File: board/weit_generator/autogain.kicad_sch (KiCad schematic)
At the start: 19 parts, among them Q1 BC547

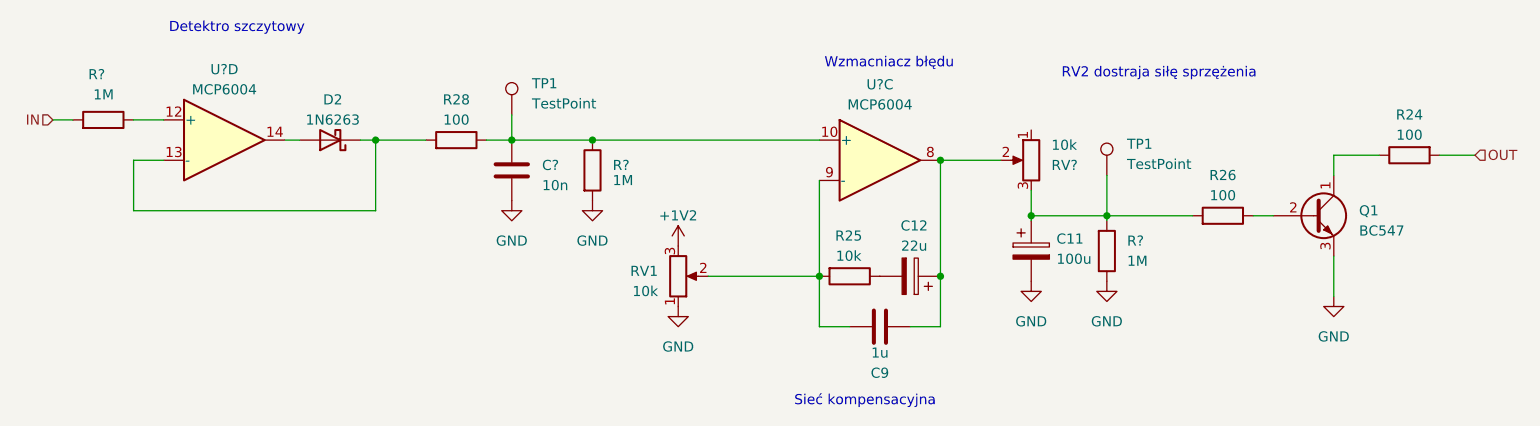
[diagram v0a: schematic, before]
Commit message: Final revision - submitting
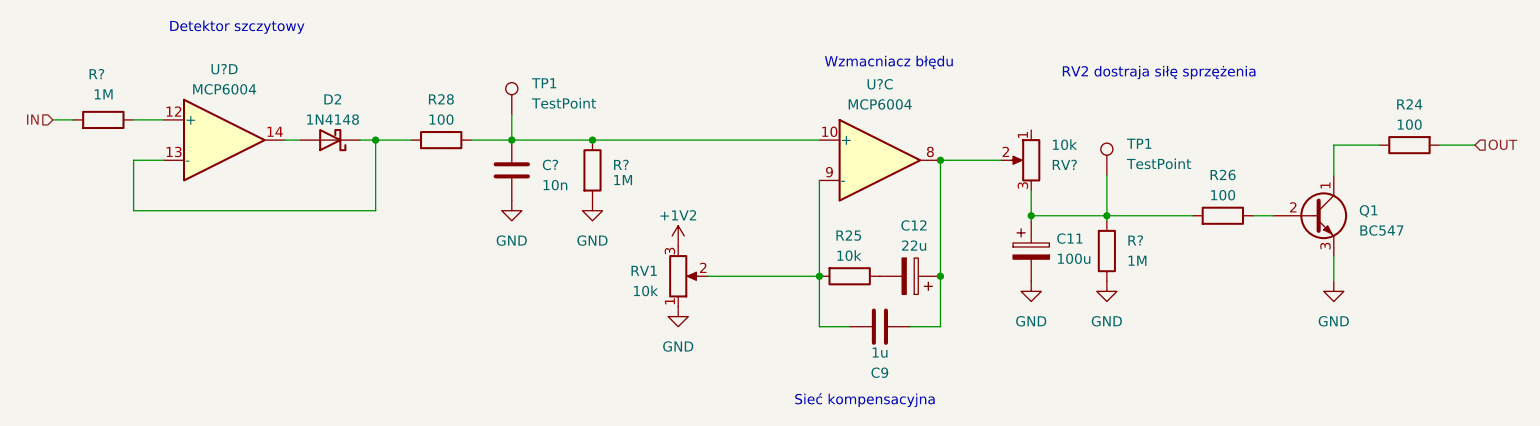
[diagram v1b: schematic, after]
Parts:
- D2: value 1N6263 -> 1N4148
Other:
- note added: "Detektor szczytowy"
- note removed: "Detektro szczytowy"
- moved on the sheet: R24, R28
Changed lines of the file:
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@@
     (stroke (width 0) (type default))
   )
-  (wire (pts (xy 234.315 97.155) (xy 238.76 97.155))
+  (wire (pts (xy 234.315 95.885) (xy 238.76 95.885))
     (stroke (width 0) (type default))
   )
@@
     (stroke (width 0) (type default))
   )
-  (wire (pts (xy 220.98 97.155) (xy 220.98 99.695))
-    (stroke (width 0) (type default))
-  )
-  (wire (pts (xy 220.98 114.935) (xy 220.98 109.855))
+  (wire (pts (xy 220.98 95.885) (xy 220.98 99.695))
+    (stroke (width 0) (type default))
+  )
+  (wire (pts (xy 220.98 113.03) (xy 220.98 109.855))
     (stroke (width 0) (type default))
   )
@@
     (stroke (width 0) (type default))
   )
-  (wire (pts (xy 100.33 95.25) (xy 106.68 95.25))
-    (stroke (width 0) (type default))
-  )
-  (wire (pts (xy 114.3 95.25) (xy 117.475 95.25))
+  (wire (pts (xy 100.33 95.25) (xy 104.775 95.25))
+    (stroke (width 0) (type default))
+  )
+  (wire (pts (xy 112.395 95.25) (xy 117.475 95.25))
     (stroke (width 0) (type default))
   )
@@
     (stroke (width 0) (type default))
   )
-  (wire (pts (xy 226.695 97.155) (xy 220.98 97.155))
+  (wire (pts (xy 226.695 95.885) (xy 220.98 95.885))
     (stroke (width 0) (type default))
   )
@@
     (effects (font (size 1.27 1.27)) (justify left bottom))
   )
-  (text "Detektro szczytowy\n" (at 74.295 81.915 0)
+  (text "Detektor szczytowy\n" (at 74.295 81.915 0)
     (effects (font (size 1.27 1.27)) (justify left bottom))
   )
-  (hierarchical_label "OUT" (shape input) (at 238.76 97.155 0) (fields_autoplaced)
+  (hierarchical_label "OUT" (shape input) (at 238.76 95.885 0) (fields_autoplaced)
     (effects (font (size 1.27 1.27)) (justify left))
   )
@@
       (effects (font (size 1.27 1.27)))
     )
-    (property "Value" "1N6263" (at 94.9325 92.71 0)
+    (property "Value" "1N4148" (at 94.9325 92.71 0)
       (effects (font (size 1.27 1.27)))
     )
@@
     )
     (property "Datasheet" "www.st.com/resource/en/datasheet/1n6263.pdf" (at 94.615 95.25 0)
+      (effects (font (size 1.27 1.27)) hide)
+    )
+    (property "Field4" "" (at 94.615 95.25 0)
       (effects (font (size 1.27 1.27)) hide)
     )
@@
     )
   )
-  (symbol (lib_id "Device:R") (at 110.49 95.25 270) (mirror x) (unit 1)
-    (in_bom yes) (on_board yes) (dnp no)
-    (property "Reference" "R28" (at 110.49 90.17 90)
-      (effects (font (size 1.27 1.27)))
-    )
-    (property "Value" "100" (at 110.49 92.71 90)
-      (effects (font (size 1.27 1.27)))
-    )
-    (property "Footprint" "Resistor_THT:R_Axial_DIN0207_L6.3mm_D2.5mm_P2.54mm_Vertical" (at 110.49 97.028 90)
-      (effects (font (size 1.27 1.27)) hide)
-    )
-    (property "Datasheet" "~" (at 110.49 95.25 0)
+  (symbol (lib_id "Device:R") (at 108.585 95.25 270) (mirror x) (unit 1)
+    (in_bom yes) (on_board yes) (dnp no)
+    (property "Reference" "R28" (at 108.585 90.17 90)
+      (effects (font (size 1.27 1.27)))
+    )
+    (property "Value" "100" (at 108.585 92.71 90)
+      (effects (font (size 1.27 1.27)))
+    )
+    (property "Footprint" "Resistor_THT:R_Axial_DIN0207_L6.3mm_D2.5mm_P2.54mm_Vertical" (at 108.585 97.028 90)
+      (effects (font (size 1.27 1.27)) hide)
+    )
+    (property "Datasheet" "~" (at 108.585 95.25 0)
       (effects (font (size 1.27 1.27)) hide)
     )
@@
     )
   )
-  (symbol (lib_id "Device:R") (at 230.505 97.155 90) (mirror x) (unit 1)
-    (in_bom yes) (on_board yes) (dnp no)
-    (property "Reference" "R24" (at 230.505 92.075 90)
-      (effects (font (size 1.27 1.27)))
-    )
-    (property "Value" "100" (at 230.505 94.615 90)
-      (effects (font (size 1.27 1.27)))
-    )
-    (property "Footprint" "Resistor_THT:R_Axial_DIN0207_L6.3mm_D2.5mm_P2.54mm_Vertical" (at 230.505 95.377 90)
-      (effects (font (size 1.27 1.27)) hide)
-    )
-    (property "Datasheet" "~" (at 230.505 97.155 0)
+  (symbol (lib_id "Device:R") (at 230.505 95.885 90) (mirror x) (unit 1)
+    (in_bom yes) (on_board yes) (dnp no)
+    (property "Reference" "R24" (at 230.505 90.805 90)
+      (effects (font (size 1.27 1.27)))
+    )
+    (property "Value" "100" (at 230.505 93.345 90)
+      (effects (font (size 1.27 1.27)))
+    )
+    (property "Footprint" "Resistor_THT:R_Axial_DIN0207_L6.3mm_D2.5mm_P2.54mm_Vertical" (at 230.505 94.107 90)
+      (effects (font (size 1.27 1.27)) hide)
+    )
+    (property "Datasheet" "~" (at 230.505 95.885 0)
       (effects (font (size 1.27 1.27)) hide)
     )
@@
     )
   )
-  (symbol (lib_id "power:GND") (at 220.98 114.935 0) (unit 1)
-    (in_bom yes) (on_board yes) (dnp no) (fields_autoplaced)
-    (property "Reference" "#PWR039" (at 220.98 121.285 0)
-      (effects (font (size 1.27 1.27)) hide)
-    )
-    (property "Value" "GND" (at 220.98 120.015 0)
-      (effects (font (size 1.27 1.27)))
-    )
-    (property "Footprint" "" (at 220.98 114.935 0)
-      (effects (font (size 1.27 1.27)) hide)
-    )
-    (property "Datasheet" "" (at 220.98 114.935 0)
-      (effects (font (size 1.27 1.27)) hide)
-    )
+  (symbol (lib_id "power:GND") (at 220.98 113.03 0) (unit 1)
+    (in_bom yes) (on_board yes) (dnp no) (fields_autoplaced)
+    (property "Reference" "#PWR039" (at 220.98 119.38 0)
+      (effects (font (size 1.27 1.27)) hide)
+    )
+    (property "Value" "GND" (at 220.98 118.11 0)
+      (effects (font (size 1.27 1.27)))
+    )
+    (property "Footprint" "" (at 220.98 113.03 0)
+      (effects (font (size 1.27 1.27)) hide)
+    )
+    (property "Datasheet" "" (at 220.98 113.03 0)
+      (effects (font (size 1.27 1.27)) hide)
+    )
